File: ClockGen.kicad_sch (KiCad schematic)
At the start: 21 parts, among them Q1 2N4258, Q2 2N4258, Y1 XT0001

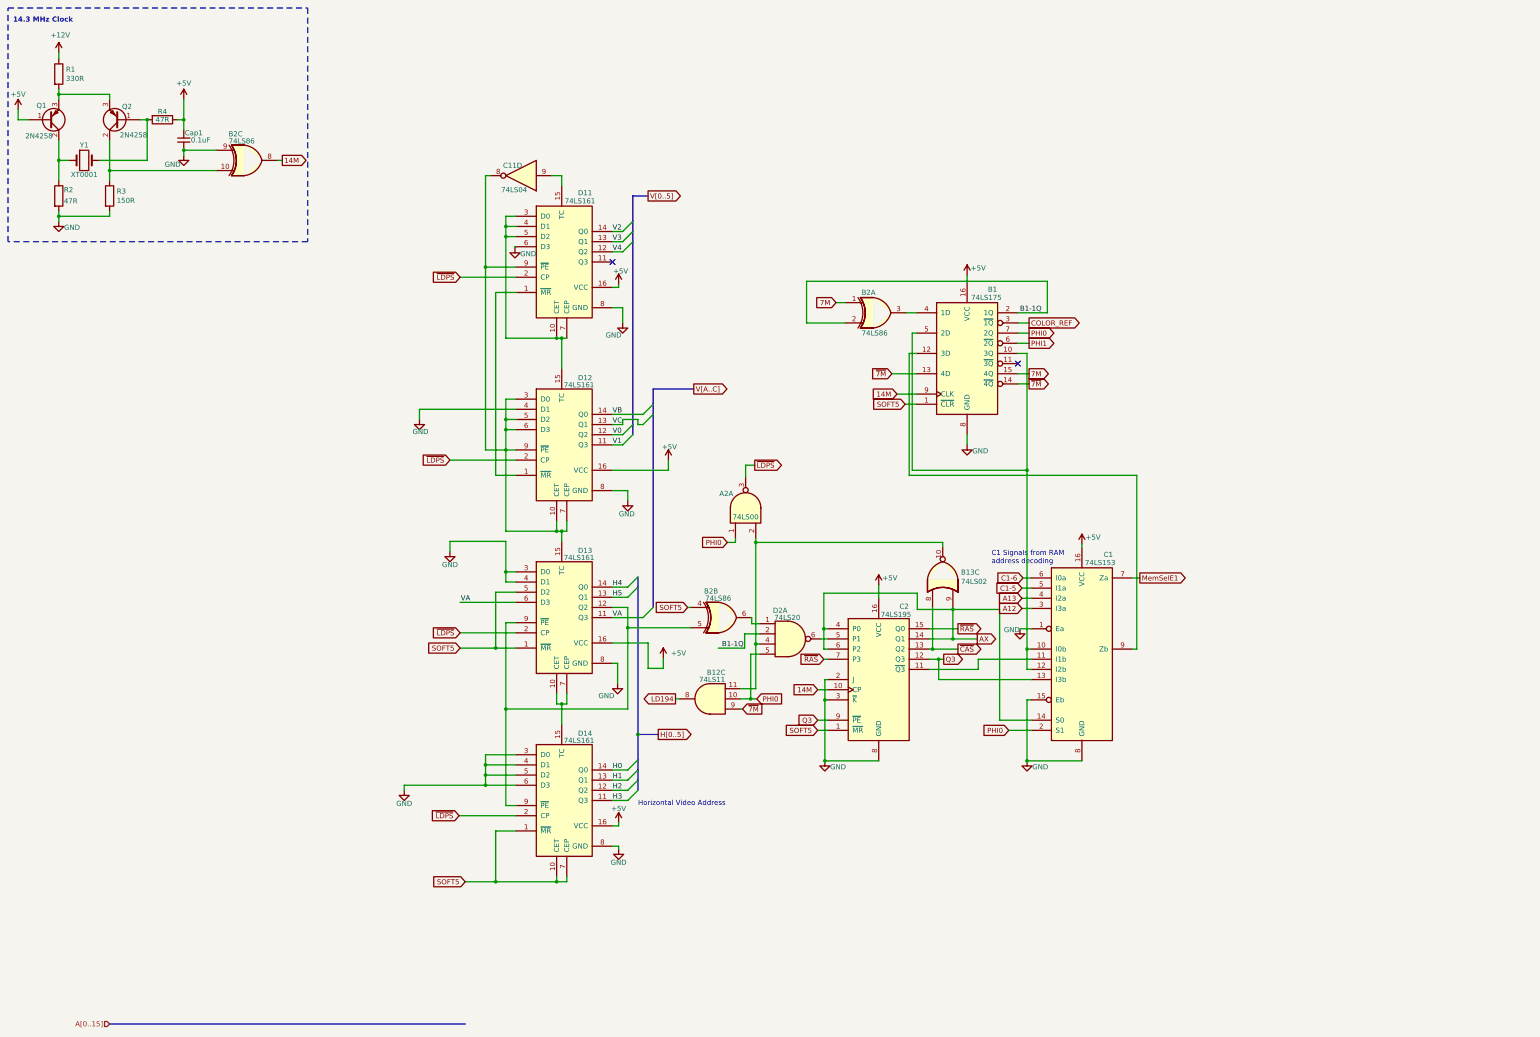
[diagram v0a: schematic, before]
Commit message: Add files via upload
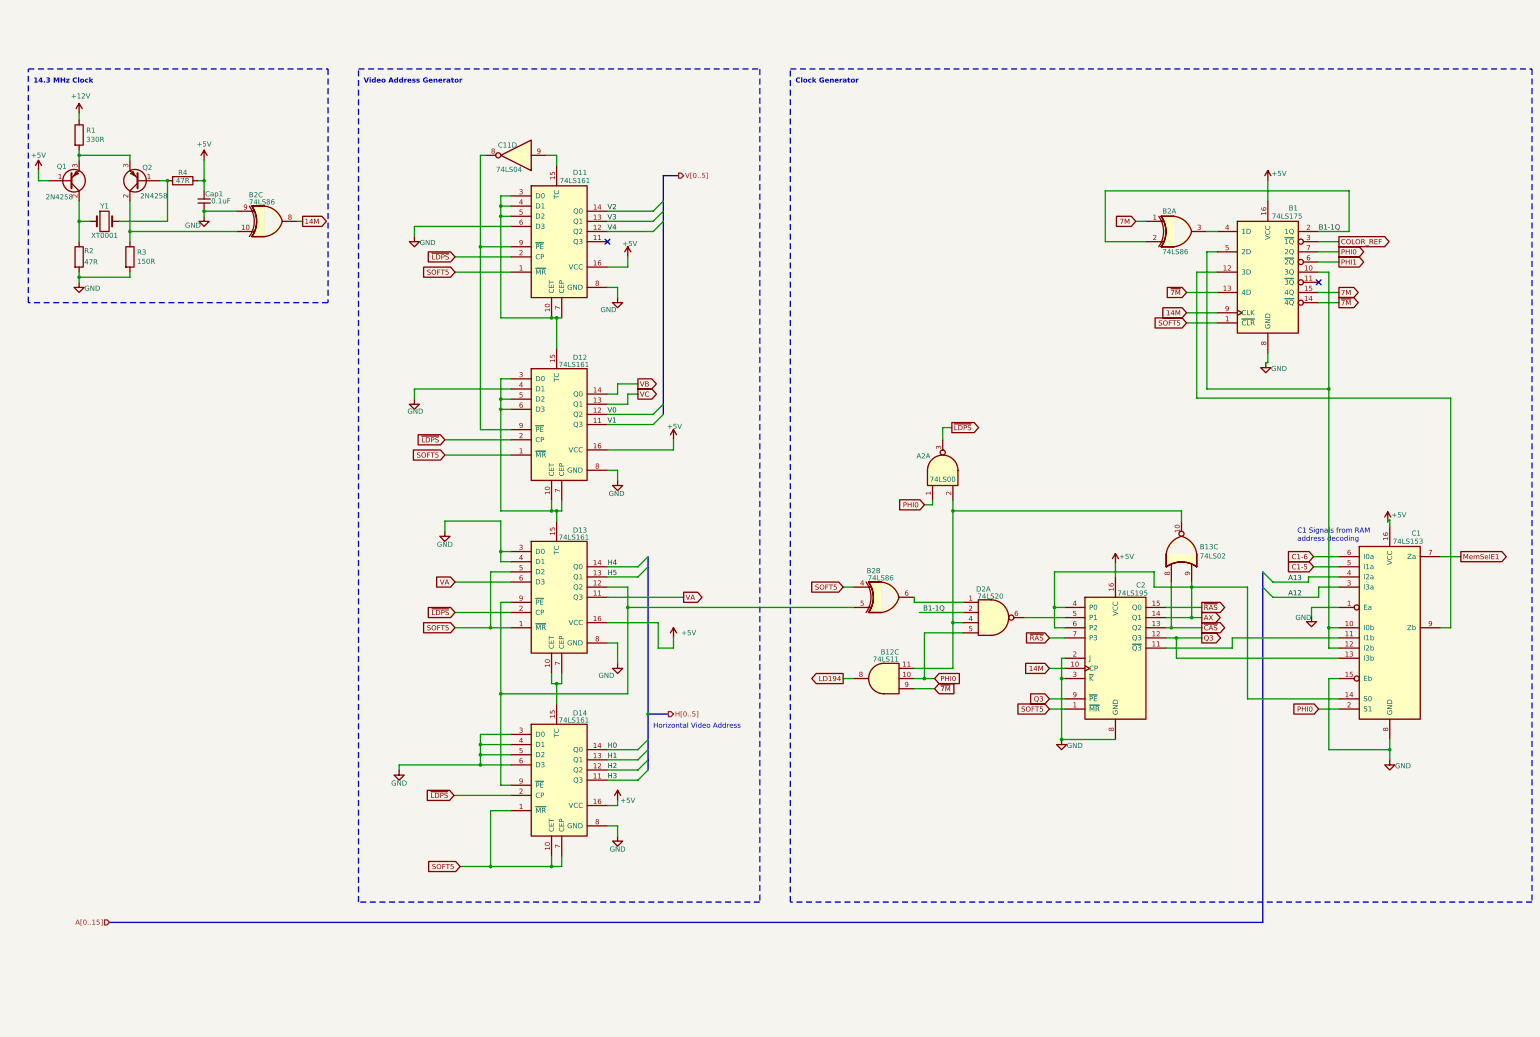
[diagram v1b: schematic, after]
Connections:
- net SOFT5: now also D11.1 (~{MR}), D12.1 (~{MR})
- net at D12.10 (CET), D12.3 (D0), D12.5 (D2)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: no longer C11.8, D11.9 (~{PE}), D12.9 (~{PE})
- new net: C11.8, D11.9 (~{PE}), D12.9 (~{PE})
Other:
- note added: "Clock Generator"
- note added: "Video Address Generator"
- moved on the sheet: A2A, B1, B12C, B13C, B2A, B2B, B2C, C1, C11D, C2, Cap1, D11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
